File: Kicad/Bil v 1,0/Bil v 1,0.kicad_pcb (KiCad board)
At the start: 2 copper layers, 100 x 75 mm, 14 parts, among them J1 Analog, J2 Digital, J3 Lidar_sensor_adafruit_VL53L0X, J4 Lidar_sensor_adafruit_VL53L0X, J5 Conn_01x04, J6 Lidar_sensor_adafruit_VL53L0X, M1 Motor_DC, M2 Motor_Servo, M4 Motor_DC

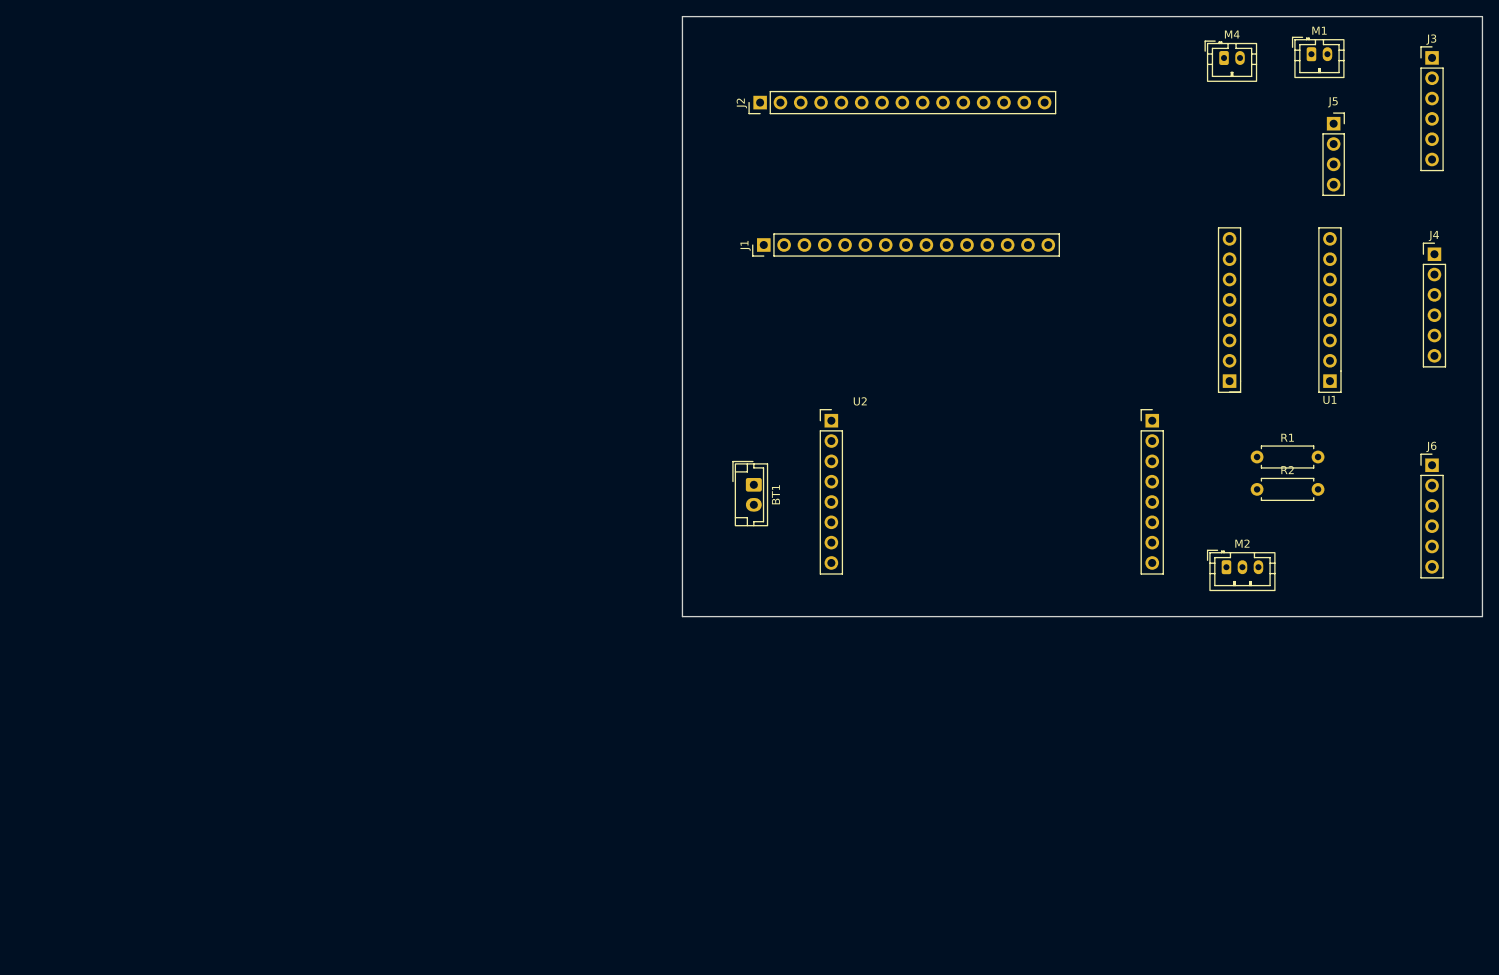
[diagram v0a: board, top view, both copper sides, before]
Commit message: 1.3 updated layout
the probably final board layout, now with power switch
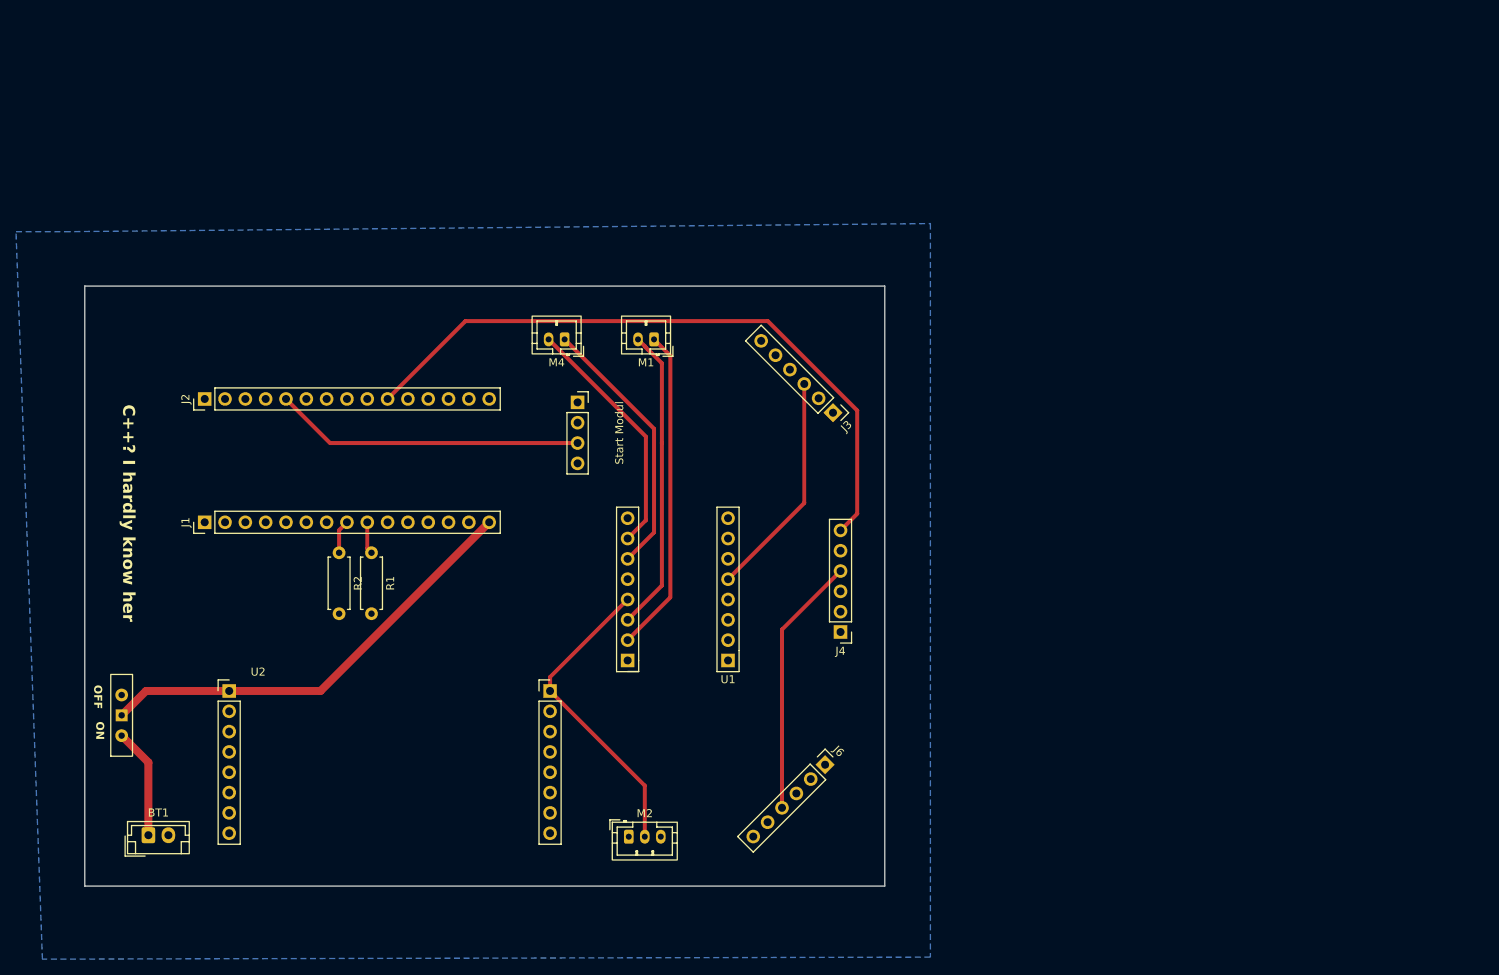
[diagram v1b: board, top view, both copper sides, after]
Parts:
- added SW2: power switch, Button_Switch_THT:SW_Slide-03_Wuerth-WS-SLTV_10x2.5x6.4_P2.54mm, F.Cu at (104.9, 110.5)
- Start Modul: renamed from J5
- moved R2 115.0 mm to (132.1, 90.2), turned to -90 degrees
- moved R1 111.3 mm to (136.1, 90.2), turned to -90 degrees
- moved Start Modul 100.7 mm to (161.9, 71.4)
- moved M4 89.6 mm to (160.3, 63.5), turned to 180 degrees
- moved M1 89.6 mm to (171.4, 63.5), turned to 180 degrees
- moved J4 88.0 mm to (194.8, 100.1), turned to 180 degrees
- moved BT1 87.4 mm to (108.2, 125.5), turned to 0 degrees
- moved J3 87.0 mm to (193.8, 72.7), turned to -135 degrees
- moved J6 84.6 mm to (192.8, 116.7), turned to -45 degrees
- moved U1 82.9 mm to (180.7, 103.6)
- moved U2 82.5 mm to (158.5, 107.4)
- moved M2 82.0 mm to (168.3, 125.7)
- moved J2 78.7 mm to (115.3, 70.9)
- moved J1 78.0 mm to (115.3, 86.4)
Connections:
- BT1 pad 1: VCC -> Net-(BT1-+)
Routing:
- net /A4/SDA: track 0.00 -> 133.7 mm
- net /A5/SCL: track 0.00 -> 125.2 mm
- net /*D5: track 0.00 -> 118.8 mm
- net /*D9: track 0.00 -> 100.8 mm
- net /*D3: track 0.00 -> 83.2 mm
- net VCC: track 0.00 -> 55.9 mm
- net /D4: track 0.00 -> 52.2 mm
- net /M1 +: track 0.00 -> 40.6 mm
- net /D8: track 0.00 -> 38.7 mm
- net /DC-DC out: track 0.00 -> 38.6 mm
- net /M1 -: track 0.00 -> 38.1 mm
- net /M2 +: track 0.00 -> 33.4 mm
- net /M2 -: track 0.00 -> 30.9 mm
- net Net-(BT1-+): track 0.00 -> 13.8 mm
- added copper zone on In2.Cu, net +3V3
- added copper zone on B.Cu, net GND
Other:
- copper layers 2 -> 4
- board text added: "C++? I hardly know her"
- board text added: "OFF"
- board text added: "ON"
